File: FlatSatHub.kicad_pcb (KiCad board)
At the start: 4 copper layers, 129.3 x 129.3 mm, 34 parts, among them J1 Jack-DC, J10 DB26_Male_HighDensity_Mountin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, J11 Conn_02x02_Odd_Even, J12 DB26_Male_HighDensity_Mountin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, J13 Conn_02x02_Odd_Even, J14 DB26_Male_HighDensity_Mountin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, J15 Conn_02x02_Odd_Even, J16 DB26_Male_HighDensity_Mountin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, J17 Conn_02x02_Odd_Even, J2 DB26_Male_HighDensity_Mountin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, J3 Conn_02x02_Odd_Even, J4 DB26_Male_HighDensity_Mountin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, J5 Conn_02x02_Odd_Even, J6 DB26_Male_HighDensity_Mountin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, J7 Conn_02x02_Odd_Even, J8 DB26_Male_HighDensity_Mountin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, J9 Conn_02x02_Odd_Even, SW1 SW_DIP_x03, SW2 SW_DIP_x03, SW3 SW_DIP_x03, SW4 SW_DIP_x03, SW5 SW_DIP_x03, SW6 SW_DIP_x03, SW7 SW_DIP_x03, SW8 SW_DIP_x03, SW9 SW_DIP_x03

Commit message: try improving positionning
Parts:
- removed R1, R2: R, Resistor_SMD:R_0603_1608Metric_Pad1.05x0.95mm_HandSolder
- added SW10: SW_SPDT, Button_Switch_SMD:SW_SPDT_PCM12, F.Cu at (83.8, 131.4)
- added SW11: SW_SPDT, Button_Switch_SMD:SW_SPDT_PCM12, F.Cu at (103.2, 131.4)
- J10, J12, J14, J16, J2, J4, J6, J8: footprint Connector_Dsub:DSUB-26-HD_Male_Horizontal_P2.29x1.98mm_EdgePinOffset3.03mm_Housed_MountingHolesOffset4.94mm -> DB-HD-26:DSUB-26-HD_Male_Horizontal_P2.29x1.98mm_EdgePinOffset3.03mm_Housed_MountingHolesOffset4.94mm_custom
- SW1: value SW_DIP_x03 -> SW_SPDT; footprint Button_Switch_THT:SW_DIP_SPSTx03_Slide_9.78x9.8mm_W7.62mm_P2.54mm -> Button_Switch_SMD:SW_SPDT_PCM12
- moved J12 285.6 mm to (94.8, 171.7)
- moved J11 283.6 mm to (34.8, 101.7), turned to 90 degrees
- moved J13 277.1 mm to (94.8, 41.6)
- moved J15 267.9 mm to (52.3, 144.1), turned to 135 degrees
- moved J7 264.8 mm to (52.3, 59.2), turned to 45 degrees
- moved J16 246.3 mm to (94.8, 31.6), turned to 180 degrees
- moved J10 238.0 mm to (45.3, 52.2), turned to 225 degrees
- moved SW9 235.2 mm to (94.8, 61.6)
- moved J17 234.1 mm to (137.2, 59.2), turned to 315 degrees
- moved SW7 208.8 mm to (123.0, 73.4), turned to 135 degrees
- moved SW8 207.7 mm to (66.5, 129.9), turned to 135 degrees
- moved J4 206.6 mm to (24.8, 101.7), turned to 270 degrees
- moved J8 191.2 mm to (45.3, 151.1), turned to 315 degrees
- moved SW6 190.2 mm to (94.8, 141.7), turned to 180 degrees
- moved J9 178.5 mm to (94.8, 161.7), turned to 180 degrees
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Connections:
- C1 pad 11: /PSU_3V3_ENABLE -> Net-(C1-Pad11)
- C1 pad 7: Vbat -> /Vin
- C1 pad 8: Vbat -> /Vin
- C2 pad 5: Vbat -> /Vin
- C2 pad 6: /PSU_5V_ENABLE -> Net-(C2-Pad6)
- J1 pad 1: Net-(J1-Pad1) -> /Vin
- SW1 pad 1: Net-(J1-Pad1) -> Vbat
- SW1 pad 2: Net-(J1-Pad1) -> /Vin
- SW1 pad 3: Net-(J1-Pad1) -> Net-(SW1-Pad3)
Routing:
- net Net-(J1-Pad1): track 43.2 -> 0.00 mm
- net /5V-C-SW: track 31.3 -> 0.00 mm
- net /3V3-C-SW: track 23.1 -> 0.00 mm
- added copper zone on In2.Cu, net 3V3
- added copper zone on B.Cu, net 5V
- removed copper zone on In2.Cu, net /3V3
- removed copper zone on B.Cu, net /5V
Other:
- board size 129.3 x 129.3 mm -> 147.8 x 147.8 mm

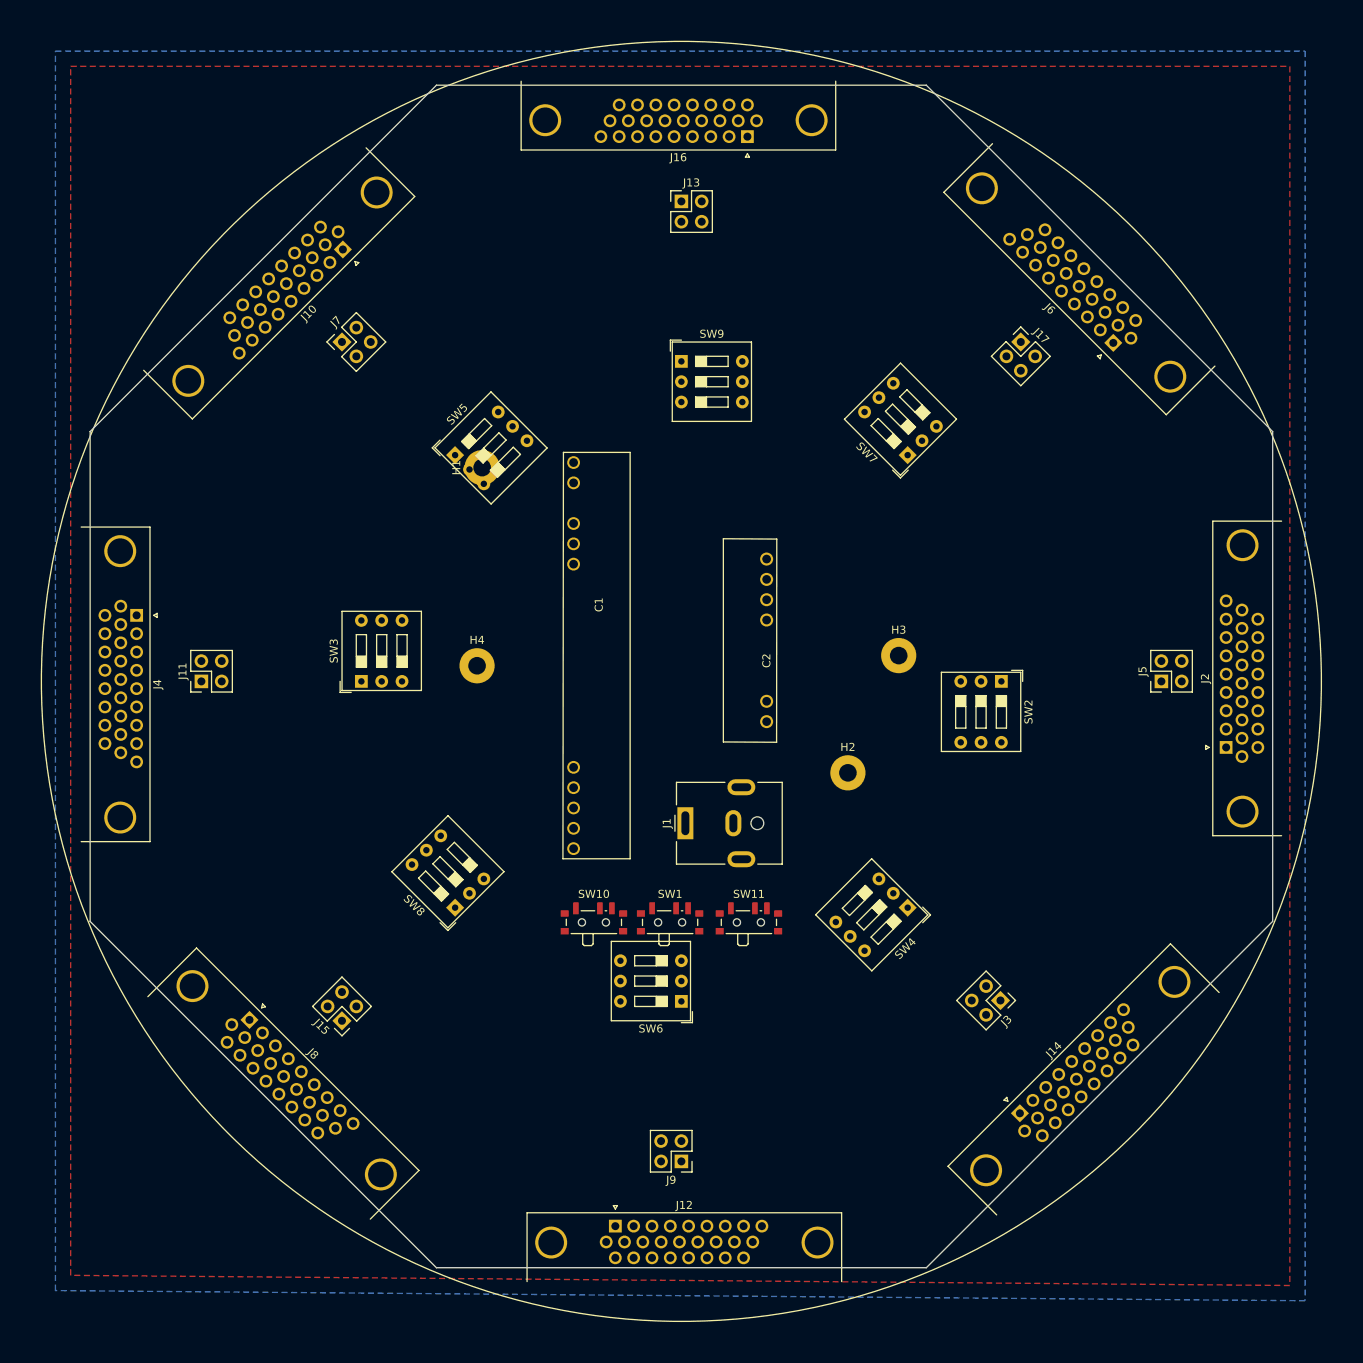
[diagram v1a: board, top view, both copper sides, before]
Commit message: re-place footprints for symmetry
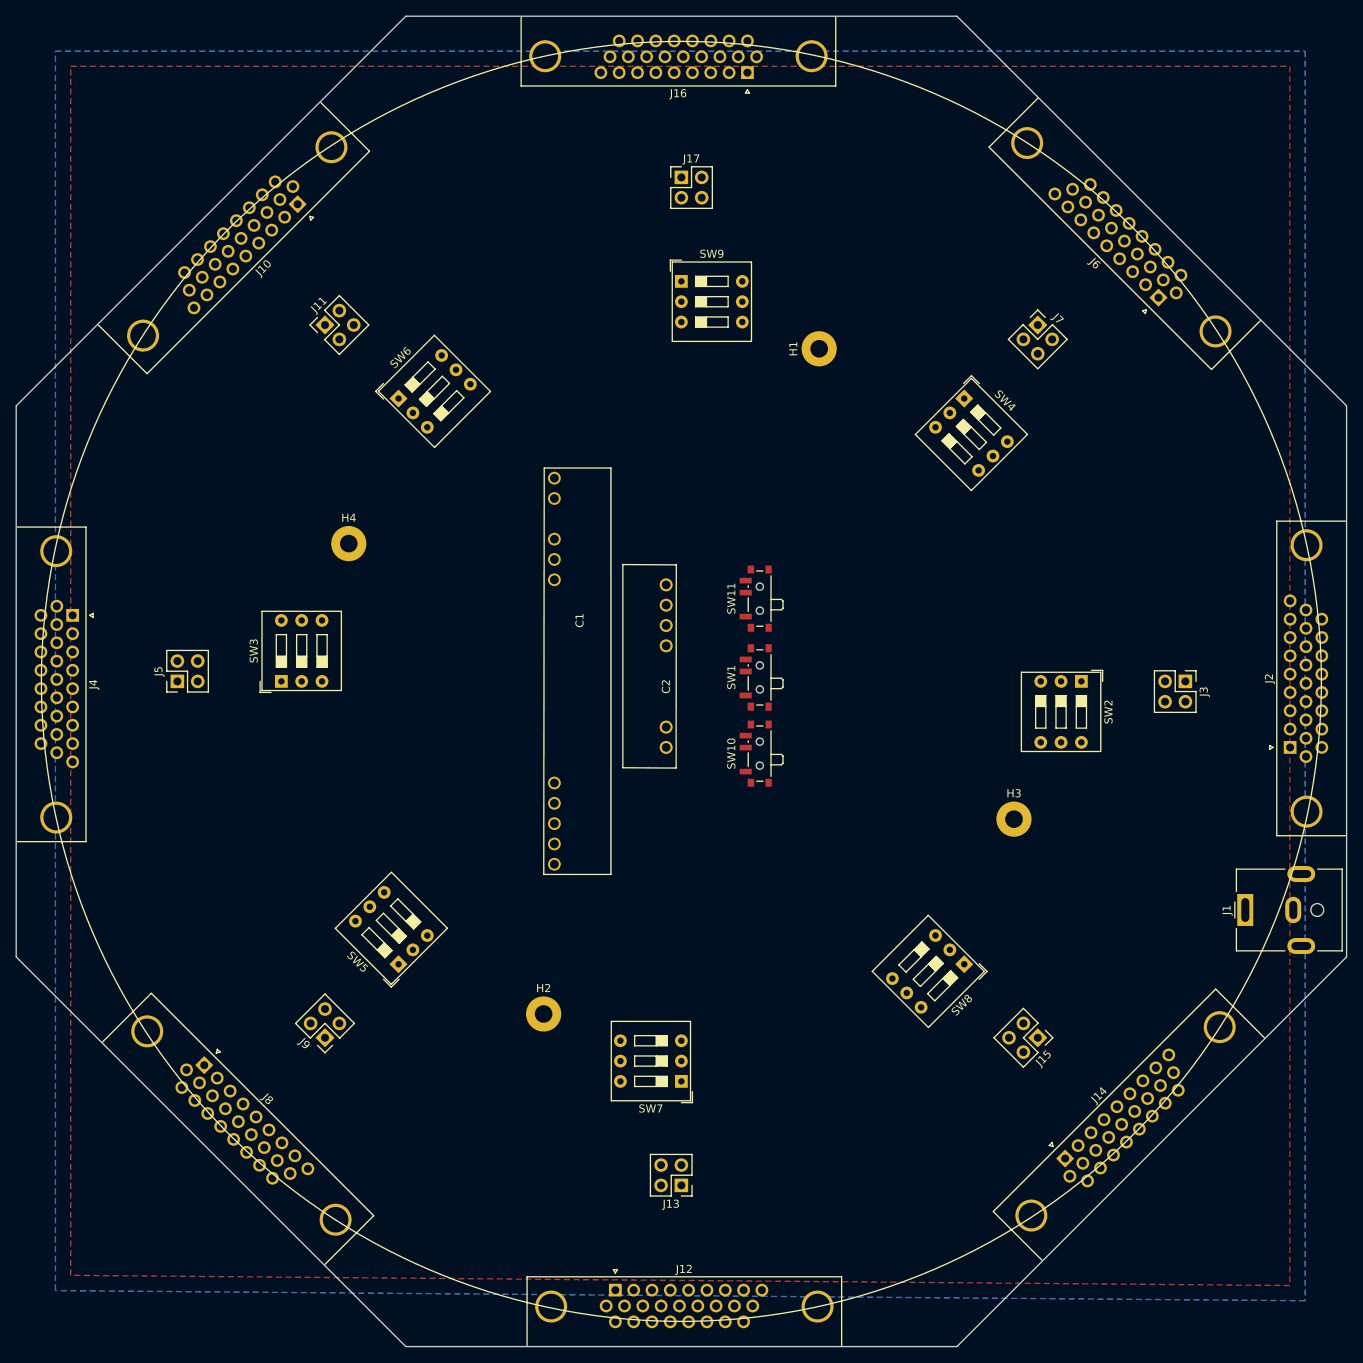
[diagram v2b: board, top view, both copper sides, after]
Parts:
- moved J13 123.0 mm to (94.8, 164.7), turned to 180 degrees
- moved J5 123.0 mm to (31.8, 101.7)
- moved J15 87.0 mm to (139.3, 146.2), turned to 225 degrees
- moved J7 87.0 mm to (139.3, 57.1), turned to 315 degrees
- moved SW6 83.2 mm to (59.4, 66.3), turned to 45 degrees
- moved SW7 83.2 mm to (94.8, 151.7), turned to 180 degrees
- moved J1 70.8 mm to (165.2, 130.2)
- moved SW8 64.0 mm to (130.1, 137.0), turned to 225 degrees
- moved SW4 64.0 mm to (130.1, 66.3), turned to 315 degrees
- moved SW5 64.0 mm to (59.4, 137.0), turned to 135 degrees
- moved H2 48.5 mm to (77.5, 143.2)
- moved J11 47.2 mm to (50.2, 57.1), turned to 45 degrees
- moved J9 47.2 mm to (50.2, 146.2), turned to 135 degrees
- moved J17 47.2 mm to (94.8, 38.6), turned to 0 degrees
- moved J3 46.1 mm to (157.8, 101.7), turned to 270 degrees
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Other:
- board size 147.8 x 147.8 mm -> 166.3 x 166.3 mm

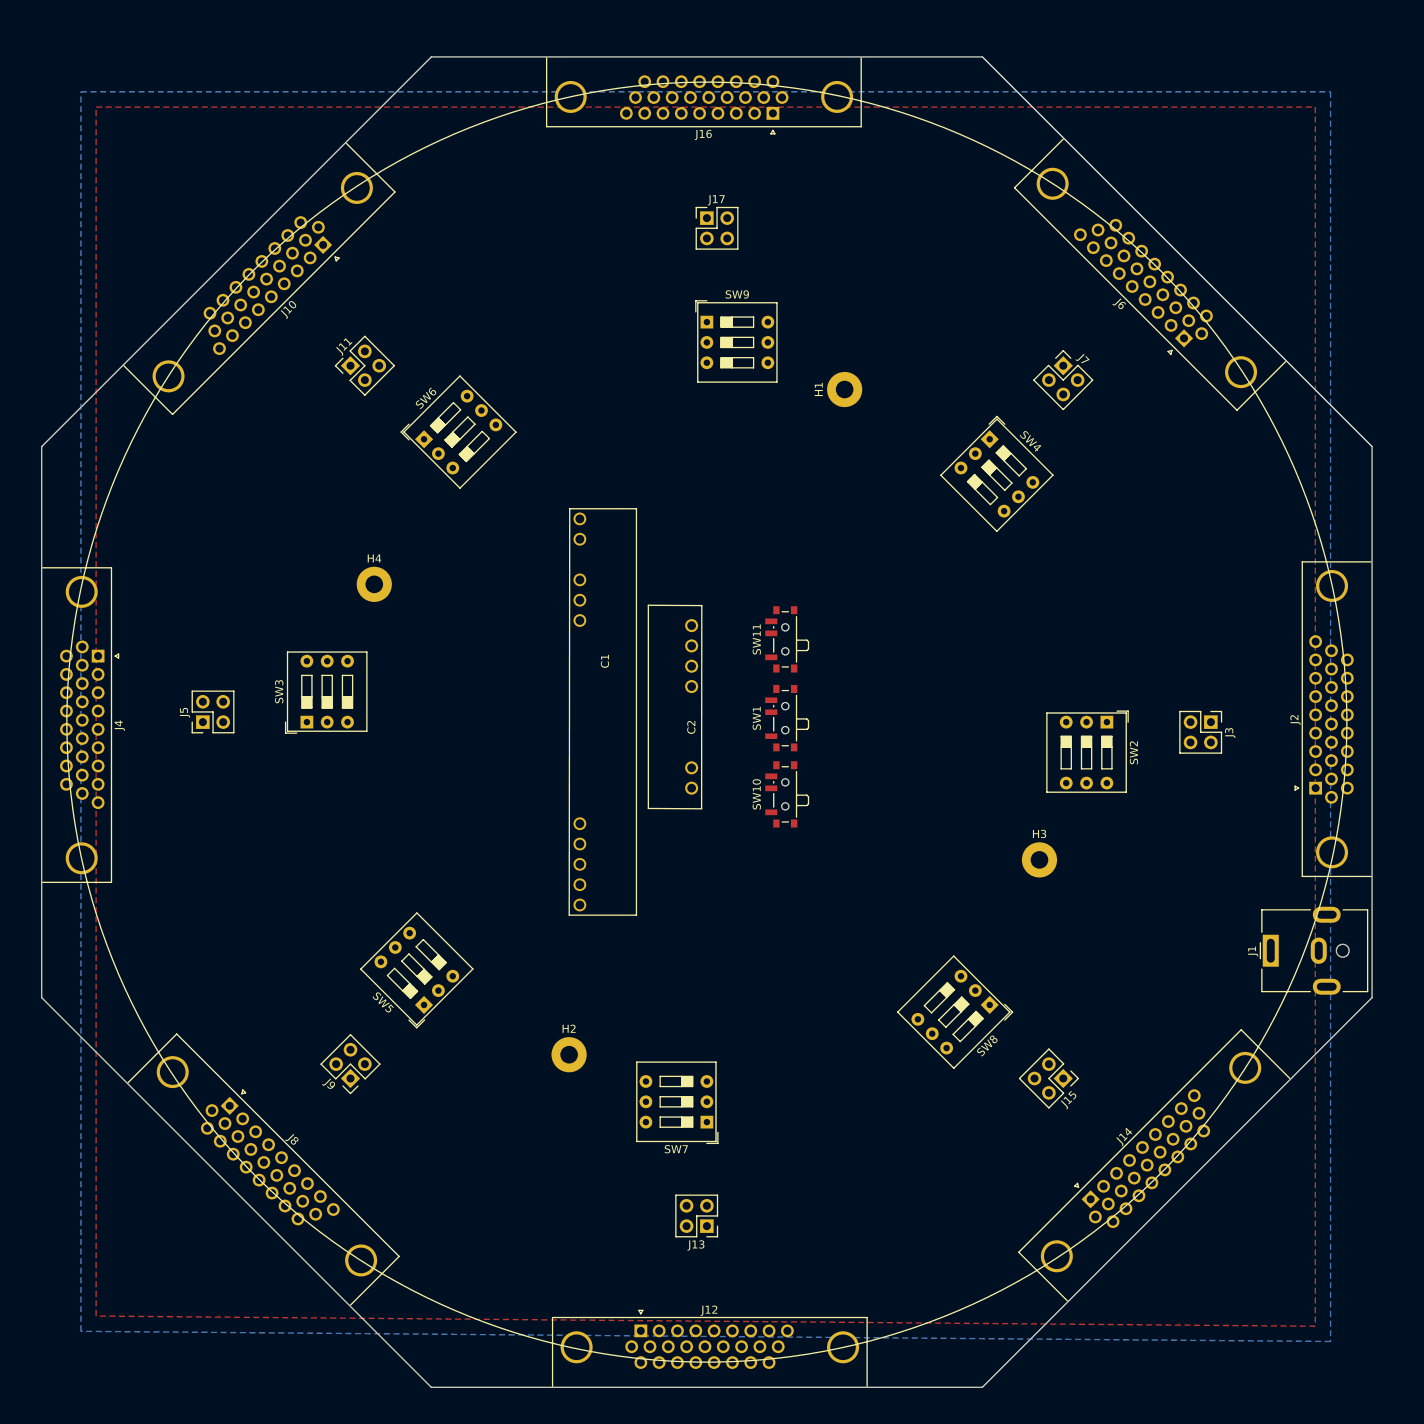
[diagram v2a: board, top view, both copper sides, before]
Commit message: minor improvements
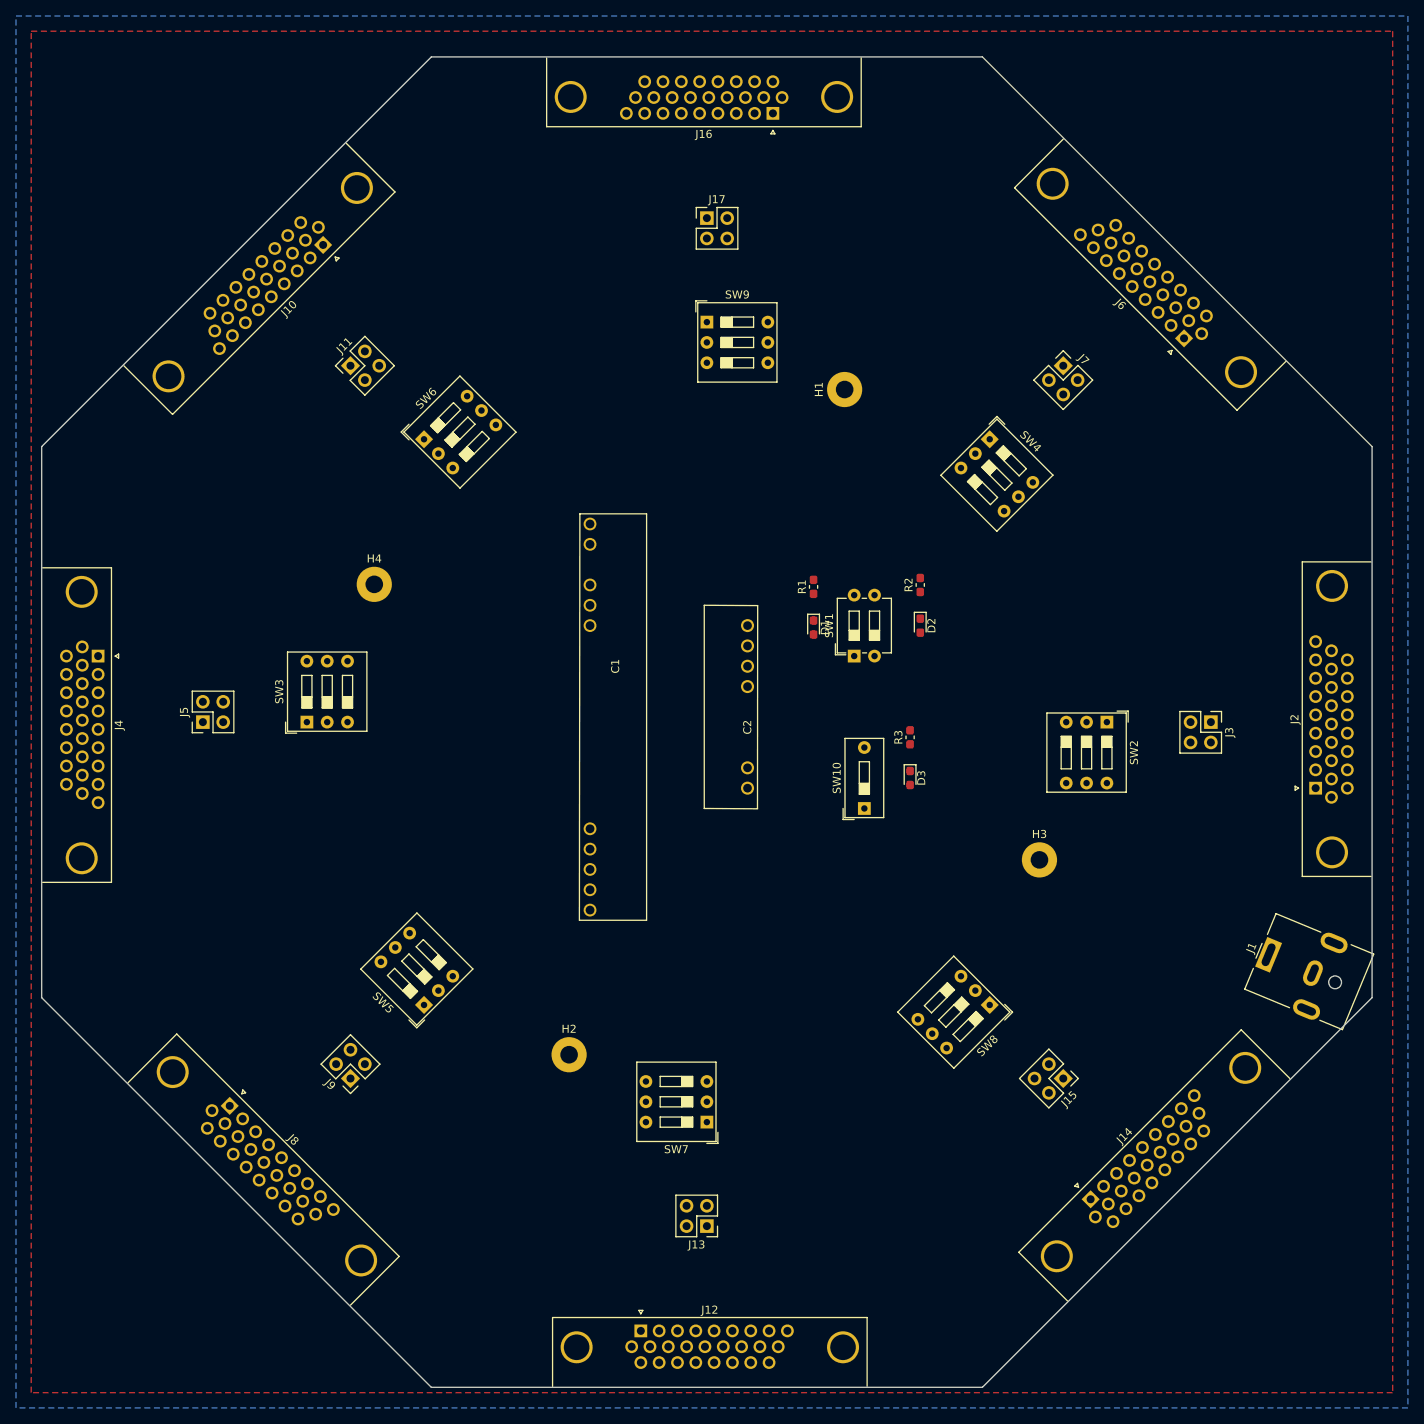
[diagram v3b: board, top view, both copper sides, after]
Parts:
- removed SW11: SW_SPDT, Button_Switch_SMD:SW_SPDT_PCM12
- added D1: GREEN LED, LED_SMD:LED_0603_1608Metric_Pad1.05x0.95mm_HandSolder, F.Cu at (108.1, 89.8)
- added D2: GREEN LED, LED_SMD:LED_0603_1608Metric_Pad1.05x0.95mm_HandSolder, F.Cu at (121.4, 89.6)
- added D3: GREEN_LED, LED_SMD:LED_0603_1608Metric_Pad1.05x0.95mm_HandSolder, F.Cu at (120.2, 108.6)
- added R1: R, Resistor_SMD:R_0603_1608Metric_Pad1.05x0.95mm_HandSolder, F.Cu at (108.1, 84.7)
- added R2: R, Resistor_SMD:R_0603_1608Metric_Pad1.05x0.95mm_HandSolder, F.Cu at (121.4, 84.5)
- added R3: R, Resistor_SMD:R_0603_1608Metric_Pad1.05x0.95mm_HandSolder, F.Cu at (120.2, 103.6)
- SW1: value SW_SPDT -> SW_DIP_x02; footprint Button_Switch_SMD:SW_SPDT_PCM12 -> Button_Switch_THT:SW_DIP_SPSTx02_Slide_6.7x6.64mm_W7.62mm_P2.54mm_LowProfile
- SW10: value SW_SPDT -> SW_SPST; footprint Button_Switch_SMD:SW_SPDT_PCM12 -> Button_Switch_THT:SW_DIP_SPSTx01_Slide_9.78x4.72mm_W7.62mm_P2.54mm
- moved SW1 11.8 mm to (113.2, 93.4)
- moved SW10 10.4 mm to (114.4, 112.4)
- moved C2 6.98 mm to (99.2, 99.7)
- moved C1 1.42 mm to (80.2, 94.7)
- moved J1 0.58 mm to (165.0, 130.7), turned to 67.5 degrees
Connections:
- SW1 pad 1: Vbat -> GND
- SW1 pad 2: /Vin -> GND
- SW1 pad 3: Net-(SW1-Pad3) -> Net-(C1-Pad11)
- SW10 pad 1: Net-(SW10-Pad1) -> /Vin
- SW10 pad 2: GND -> Vbat
